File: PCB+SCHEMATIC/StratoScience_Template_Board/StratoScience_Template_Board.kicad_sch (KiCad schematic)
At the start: 6 parts, among them J1 Arduino DC Jack (6-12v)

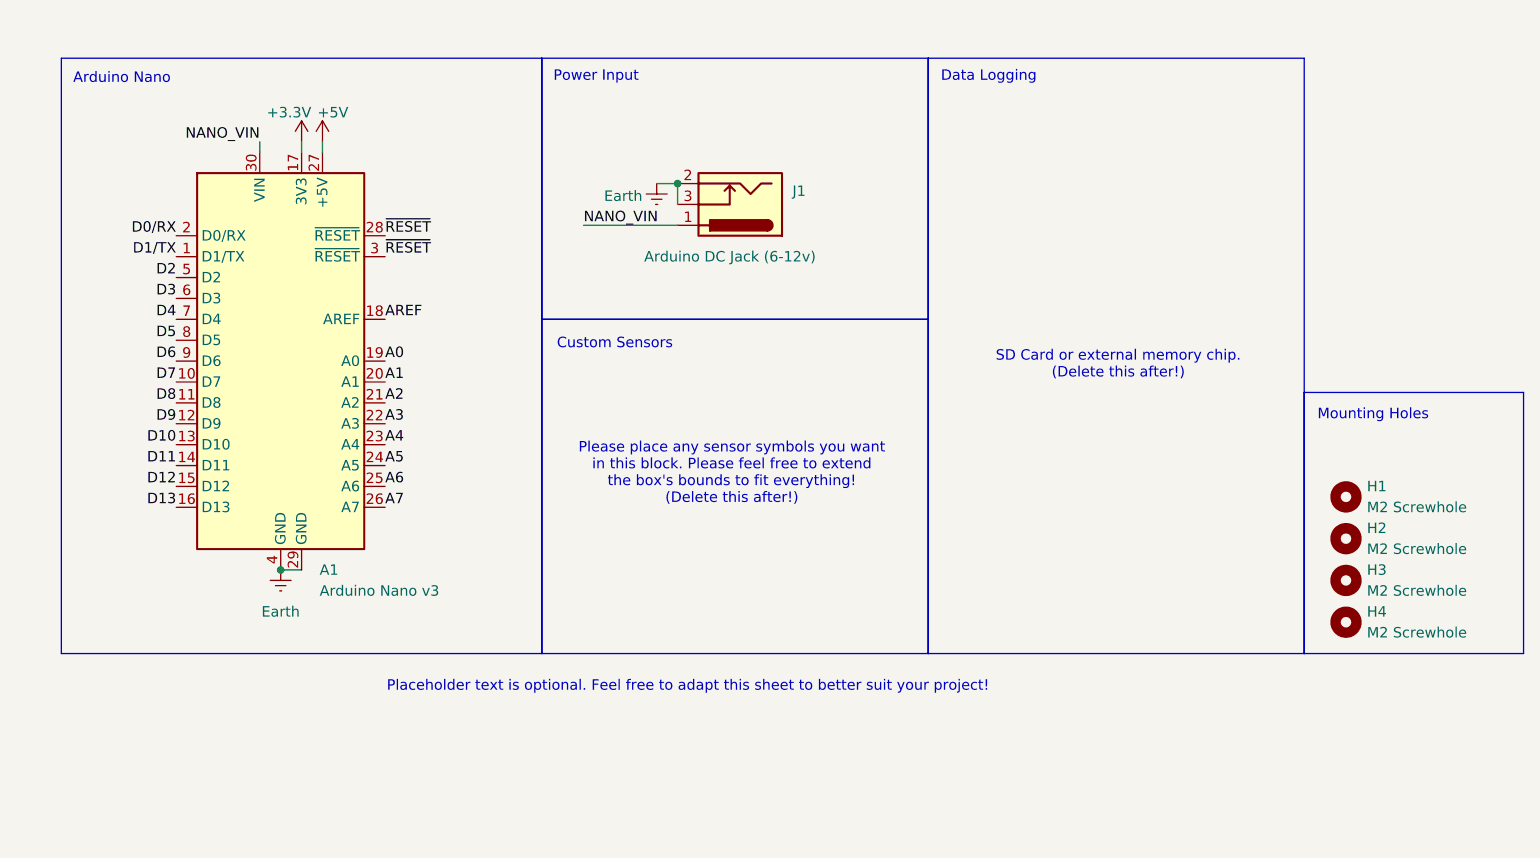
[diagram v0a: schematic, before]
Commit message: adding stuff
just adding stuff
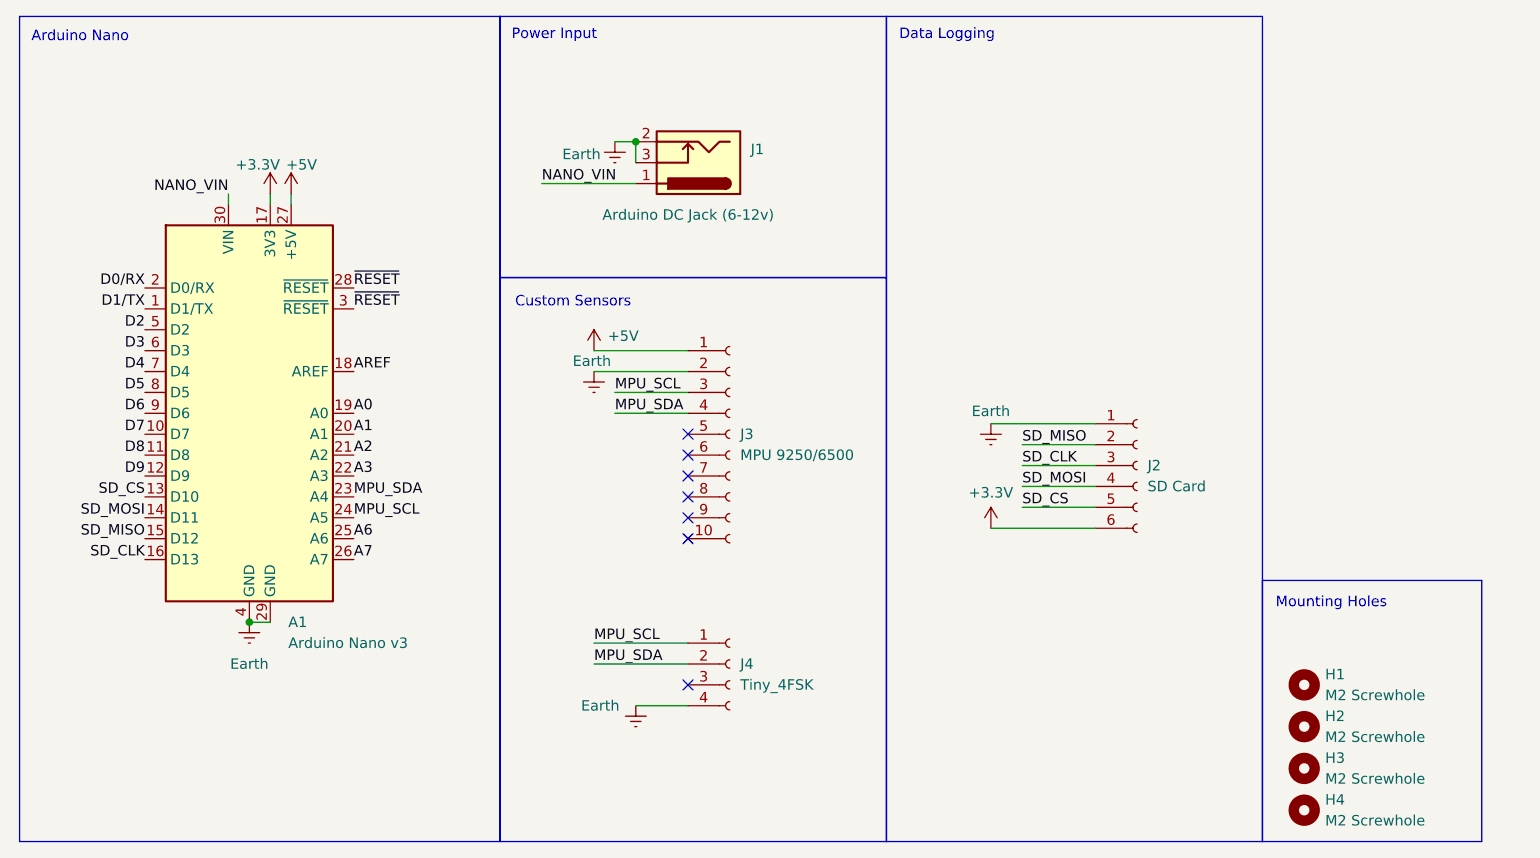
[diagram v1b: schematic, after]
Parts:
- added J2: SD Card, Connector_PinSocket_2.54mm:PinSocket_1x06_P2.54mm_Vertical, symbol Connector:Conn_01x06_Socket
- added J3: MPU 9250/6500, Connector_PinSocket_2.54mm:PinSocket_1x10_P2.54mm_Vertical, symbol Connector:Conn_01x10_Socket
- added J4: Tiny_4FSK, Connector_JST:JST_PH_B4B-PH-K_1x04_P2.00mm_Vertical, symbol Connector:Conn_01x04_Socket
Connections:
- net +3.3V: now also J2.6 (Pin_6)
- net +5V: now also J3.1 (Pin_1)
- net Earth: now also J2.1 (Pin_1), J3.2 (Pin_2), J4.4 (Pin_4)
- net A4 renamed MPU_SDA
- net MPU_SDA: now also J3.4 (Pin_4), J4.2 (Pin_2)
- net A5 renamed MPU_SCL
- net MPU_SCL: now also J3.3 (Pin_3), J4.1 (Pin_1)
- net D10 renamed SD_CS
- net SD_CS: now also J2.5 (Pin_5)
- net D11 renamed SD_MOSI
- net SD_MOSI: now also J2.4 (Pin_4)
- net D12 renamed SD_MISO
- net SD_MISO: now also J2.2 (Pin_2)
- net D13 renamed SD_CLK
- net SD_CLK: now also J2.3 (Pin_3)
- no-connect marks 0 -> 7
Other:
- note removed: "Placeholder text is optional. Feel free to adapt this sheet to better suit your project!"
- note removed: "Please place any sensor symbols you want in this block. Please feel free to extend the box's bounds to fit everything! (Delete this after!)"
- note removed: "SD Card or external memory chip. (Delete this after!)"
- title: My StratoScience Project Name (double-click here to edit) -> Nathaniel Fine's
- moved on the sheet: A1, H1, H2, H3, H4, J1
